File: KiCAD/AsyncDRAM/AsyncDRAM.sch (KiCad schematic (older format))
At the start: 6 parts

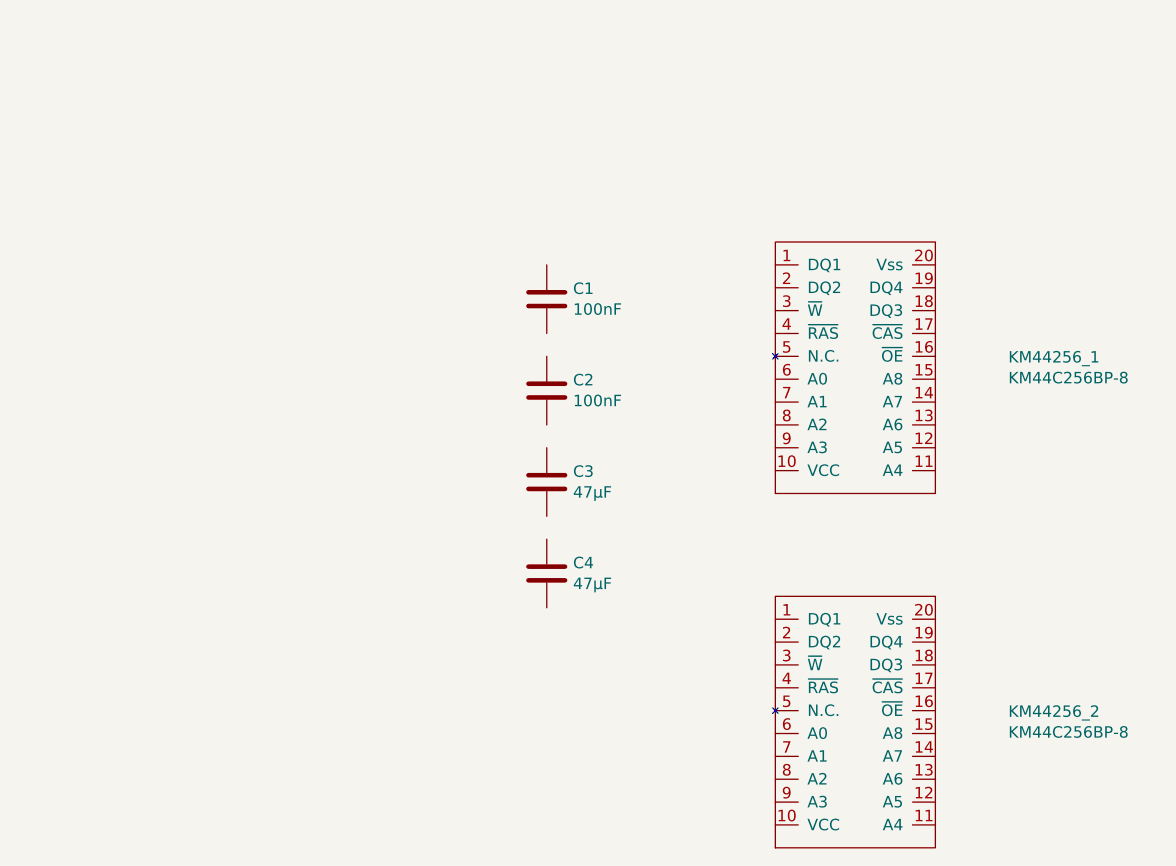
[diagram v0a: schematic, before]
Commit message: Update
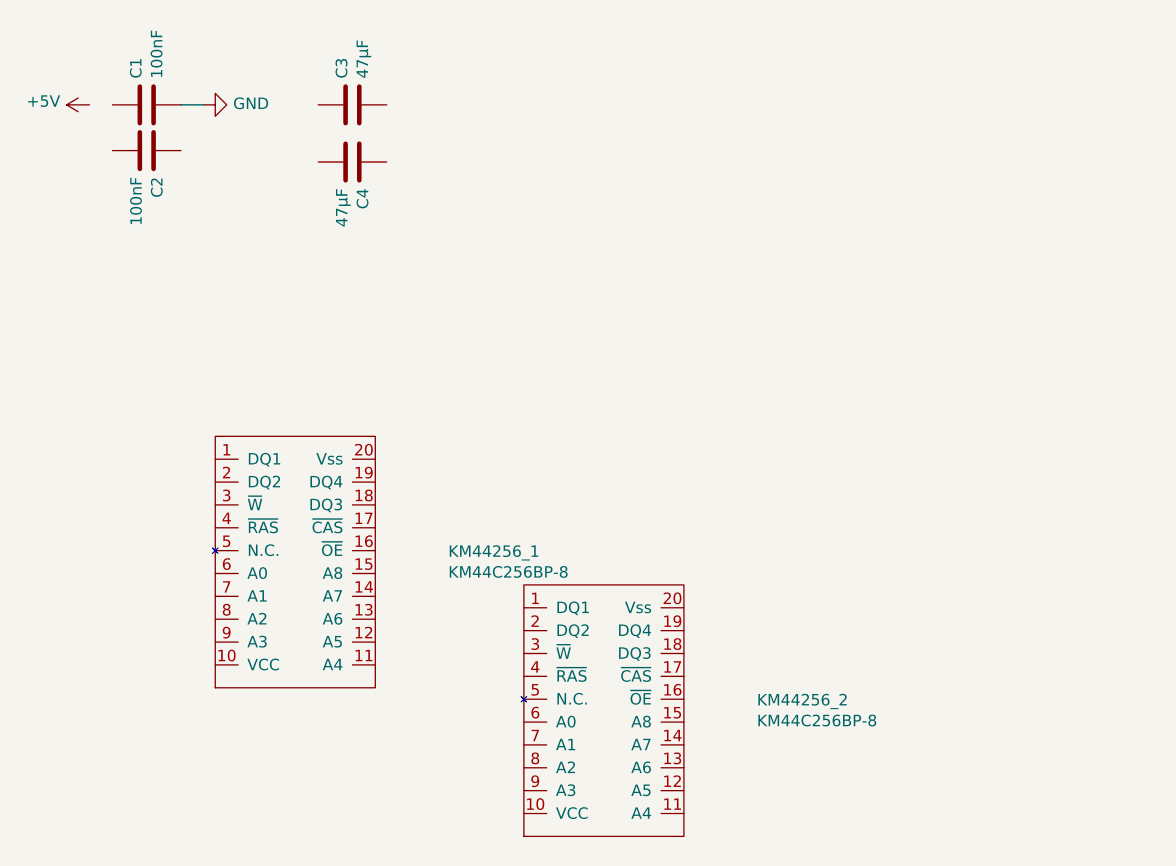
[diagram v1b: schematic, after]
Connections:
- net GND: now reaches C1.2
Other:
- moved on the sheet: C1, C2, C3, C4, KM44256_1, KM44256_2
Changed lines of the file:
@@
 EESchema Schematic File Version 4
+LIBS:AsyncDRAM-cache
 EELAYER 30 0
 EELAYER END
@@
 L MyLibrary:KM44C256BP-8 KM44256_1
 U 1 1 5DA9F5FC
-P 4200 2250
-F 0 "KM44256_1" H 4869 2296 50  0000 L CNN
-F 1 "KM44C256BP-8" H 4869 2205 50  0000 L CNN
-F 2 "DIP:DIP-20_W7.62mm" H 4150 2350 50  0001 C CNN
-F 3 "" H 4150 2350 50  0001 C CNN
-	1    4200 2250
+P 1750 3100
+F 0 "KM44256_1" H 2419 3146 50  0000 L CNN
+F 1 "KM44C256BP-8" H 2419 3055 50  0000 L CNN
+F 2 "DIP:DIP-20_W7.62mm" H 1700 3200 50  0001 C CNN
+F 3 "" H 1700 3200 50  0001 C CNN
+	1    1750 3100
 	1    0    0    -1
 $EndComp
@@
 L MyLibrary:KM44C256BP-8 KM44256_2
 U 1 1 5DA9FC1B
-P 4200 3800
-F 0 "KM44256_2" H 4869 3846 50  0000 L CNN
-F 1 "KM44C256BP-8" H 4869 3755 50  0000 L CNN
-F 2 "DIP:DIP-20_W7.62mm" H 4150 3900 50  0001 C CNN
-F 3 "" H 4150 3900 50  0001 C CNN
-	1    4200 3800
+P 3100 3750
+F 0 "KM44256_2" H 3769 3796 50  0000 L CNN
+F 1 "KM44C256BP-8" H 3769 3705 50  0000 L CNN
+F 2 "DIP:DIP-20_W7.62mm" H 3050 3850 50  0001 C CNN
+F 3 "" H 3050 3850 50  0001 C CNN
+	1    3100 3750
 	1    0    0    -1
 $EndComp
@@
 L Device:C C1
 U 1 1 5DAA5148
-P 2850 1950
-F 0 "C1" H 2965 1996 50  0000 L CNN
-F 1 "100nF" H 2965 1905 50  0000 L CNN
-F 2 "CapacitorSMD:C_0805_2012Metric" H 2888 1800 50  0001 C CNN
-F 3 "~" H 2850 1950 50  0001 C CNN
-	1    2850 1950
-	1    0    0    -1
+P 1100 1100
+F 0 "C1" H 1215 1146 50  0000 L CNN
+F 1 "100nF" H 1215 1055 50  0000 L CNN
+F 2 "CapacitorSMD:C_0805_2012Metric" H 1138 950 50  0001 C CNN
+F 3 "~" H 1100 1100 50  0001 C CNN
+	1    1100 1100
+	0    -1   -1   0
 $EndComp
 $Comp
 L Device:C C2
 U 1 1 5DAA556A
-P 2850 2350
-F 0 "C2" H 2965 2396 50  0000 L CNN
-F 1 "100nF" H 2965 2305 50  0000 L CNN
-F 2 "CapacitorSMD:C_0805_2012Metric" H 2888 2200 50  0001 C CNN
-F 3 "~" H 2850 2350 50  0001 C CNN
-	1    2850 2350
-	1    0    0    -1
+P 1100 1300
+F 0 "C2" H 1215 1346 50  0000 L CNN
+F 1 "100nF" H 1215 1255 50  0000 L CNN
+F 2 "CapacitorSMD:C_0805_2012Metric" H 1138 1150 50  0001 C CNN
+F 3 "~" H 1100 1300 50  0001 C CNN
+	1    1100 1300
+	0    1    1    0
 $EndComp
 $Comp
 L Device:C C3
 U 1 1 5DAA5879
-P 2850 2750
-F 0 "C3" H 2965 2796 50  0000 L CNN
-F 1 "47µF" H 2965 2705 50  0000 L CNN
-F 2 "CapacitorSMD:C_0805_2012Metric" H 2888 2600 50  0001 C CNN
-F 3 "~" H 2850 2750 50  0001 C CNN
-	1    2850 2750
-	1    0    0    -1
+P 2000 1100
+F 0 "C3" H 2115 1146 50  0000 L CNN
+F 1 "47µF" H 2115 1055 50  0000 L CNN
+F 2 "CapacitorSMD:C_0805_2012Metric" H 2038 950 50  0001 C CNN
+F 3 "~" H 2000 1100 50  0001 C CNN
+	1    2000 1100
+	0    -1   -1   0
 $EndComp
 $Comp
 L Device:C C4
 U 1 1 5DAA6473
-P 2850 3150
-F 0 "C4" H 2965 3196 50  0000 L CNN
-F 1 "47µF" H 2965 3105 50  0000 L CNN
-F 2 "CapacitorSMD:C_0805_2012Metric" H 2888 3000 50  0001 C CNN
-F 3 "~" H 2850 3150 50  0001 C CNN
-	1    2850 3150
-	1    0    0    -1
+P 2000 1350
+F 0 "C4" H 2115 1396 50  0000 L CNN
+F 1 "47µF" H 2115 1305 50  0000 L CNN
+F 2 "CapacitorSMD:C_0805_2012Metric" H 2038 1200 50  0001 C CNN
+F 3 "~" H 2000 1350 50  0001 C CNN
+	1    2000 1350
+	0    1    1    0
 $EndComp
+$Comp
+L Power:+5V #PWR?
+U 1 1 5DAAB244
+P 850 1100
+F 0 "#PWR?" H 850 950 50  0001 C CNN
+F 1 "+5V" V 865 1228 50  0000 L CNN
+F 2 "" H 850 1100 50  0001 C CNN
+F 3 "" H 850 1100 50  0001 C CNN
+	1    850  1100
+	0    -1   -1   0
+$EndComp
+$Comp
+L Power:GND #PWR?
+U 1 1 5DAAB9E6
+P 1350 1100
+F 0 "#PWR?" H 1350 850 50  0001 C CNN
+F 1 "GND" V 1355 972 50  0000 R CNN
+F 2 "" H 1350 1100 50  0001 C CNN
+F 3 "" H 1350 1100 50  0001 C CNN
+	1    1350 1100
+	0    -1   -1   0
+$EndComp
+Wire Wire Line
+	1250 1100 1350 1100
 $EndSCHEMATC
